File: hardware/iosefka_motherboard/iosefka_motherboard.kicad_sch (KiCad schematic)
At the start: 16 parts, among them J4 Conn_01x10, J9 Conn_01x10, U5 24LC256, U6 Raspberry Pi Pico, U7 MCP3201, U8 MCP4822

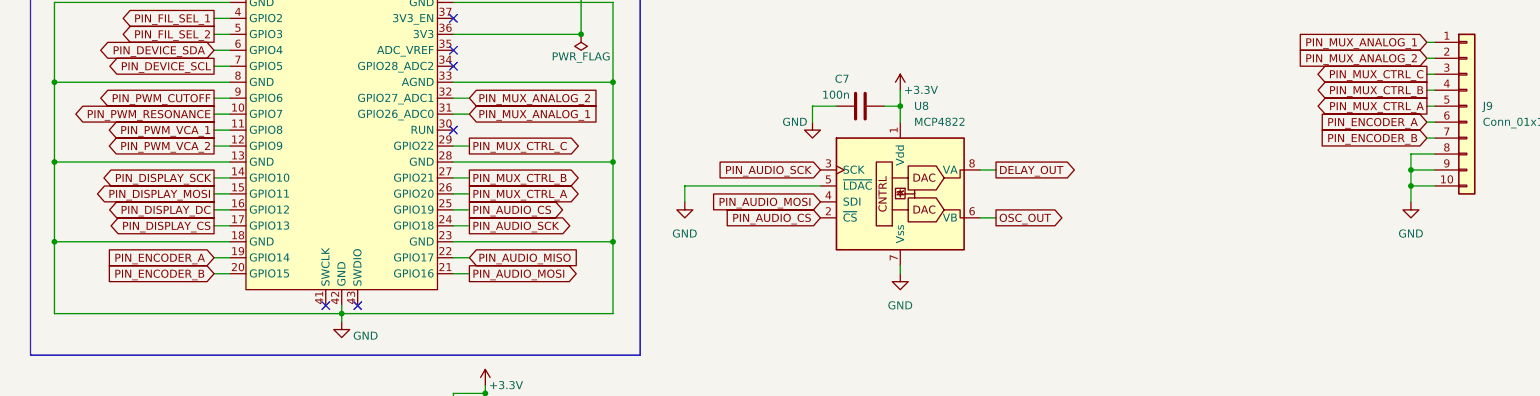
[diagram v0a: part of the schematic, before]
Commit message: added docs
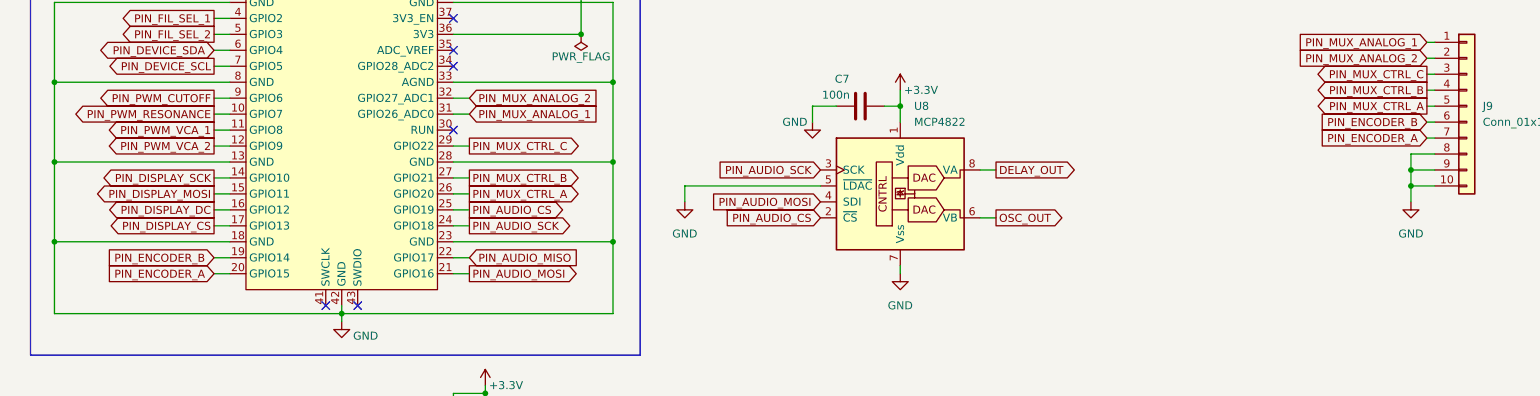
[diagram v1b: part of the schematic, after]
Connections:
- net PIN_ENCODER_A: now also J9.7 (Pin_7), U6.20 (GPIO15); no longer J9.6 (Pin_6), U6.19 (GPIO14)
- net PIN_ENCODER_B: now also J9.6 (Pin_6), U6.19 (GPIO14); no longer J9.7 (Pin_7), U6.20 (GPIO15)
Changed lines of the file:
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@@
+		)
+	)
+	(global_label "PIN_ENCODER_A"
+		(shape input)
+		(at 43.18 110.49 180)
+		(fields_autoplaced yes)
+		(effects
+			(font
+				(size 1.27 1.27)
+			)
+			(justify right)
+		)
+		(property "Intersheetrefs" "${INTERSHEET_REFS}"
+			(at 25.1967 110.49 0)
+			(effects
+				(font
+					(size 1.27 1.27)
+				)
+				(justify right)
+				(hide yes)
+			)
+		)
+	)
+	(global_label "PIN_PWM_VCA_2"
+		(shape output)
+		(at 43.18 90.17 180)
+		(fields_autoplaced yes)
+		(effects
+			(font
+				(size 1.27 1.27)
+			)
+			(justify right)
+		)
+		(property "Intersheetrefs" "${INTERSHEET_REFS}"
+			(at 25.2572 90.17 0)
+			(effects
+				(font
+					(size 1.27 1.27)
+				)
+				(justify right)
+				(hide yes)
+			)
+		)
+	)
+	(global_label "PIN_MUX_ANALOG_1"
+		(shape input)
+		(at 236.22 73.66 180)
+		(fields_autoplaced yes)
+		(effects
+			(font
+				(size 1.27 1.27)
+			)
+			(justify right)
+		)
+		(property "Intersheetrefs" "${INTERSHEET_REFS}"
+			(at 214.7895 73.66 0)
+			(effects
+				(font
+					(size 1.27 1.27)
+				)
+				(justify right)
+				(hide yes)
+			)
+		)
+	)
+	(global_label "PIN_AUDIO_SCK"
+		(shape input)
+		(at 99.06 152.4 0)
+		(fields_autoplaced yes)
+		(effects
+			(font
+				(size 1.27 1.27)
+			)
+			(justify left)
+		)
+		(property "Intersheetrefs" "${INTERSHEET_REFS}"
+			(at 116.5596 152.4 0)
+			(effects
+				(font
+					(size 1.27 1.27)
+				)
+				(justify left)
+				(hide yes)
+			)
+		)
+	)
+	(global_label "PIN_MUX_CTRL_C"
+		(shape output)
+		(at 83.82 90.17 0)
+		(fields_autoplaced yes)
+		(effects
+			(font
+				(size 1.27 1.27)
+			)
+			(justify left)
+		)
+		(property "Intersheetrefs" "${INTERSHEET_REFS}"
+			(at 102.7104 90.17 0)
+			(effects
+				(font
+					(size 1.27 1.27)
+				)
+				(justify left)
+				(hide yes)
+			)
+		)
+	)
+	(global_label "PIN_DEVICE_SCL"
+		(shape output)
+		(at 236.22 62.23 180)
+		(fields_autoplaced yes)
+		(effects
+			(font
+				(size 1.27 1.27)
+			)
+			(justify right)
+		)
+		(property "Intersheetrefs" "${INTERSHEET_REFS}"
+			(at 216.8835 62.23 0)
+			(effects
+				(font
+					(size 1.27 1.27)
+				)
+				(justify right)
+				(hide yes)
+			)
+		)
+	)
+	(global_label "PIN_DISPLAY_CS"
+		(shape output)
+		(at 43.18 102.87 180)
+		(fields_autoplaced yes)
+		(effects
+			(font
+				(size 1.27 1.27)
+			)
+			(justify right)
+		)
+		(property "Intersheetrefs" "${INTERSHEET_REFS}"
+			(at 25.0152 102.87 0)
+			(effects
+				(font
+					(size 1.27 1.27)
+				)
+				(justify right)
+				(hide yes)
+			)
+		)
+	)
+	(global_label "OSC_OUT"
+		(shape output)
+		(at 167.64 101.6 0)
+		(fields_autoplaced yes)
+		(effects
+			(font
+				(size 1.27 1.27)
+			)
+			(justify left)
+		)
+		(property "Intersheetrefs" "${INTERSHEET_REFS}"
+			(at 180.8457 101.6 0)
+			(effects
+				(font
+					(size 1.27 1.27)
+				)
+				(justify left)
+				(hide yes)
+			)
 		)
 	)
 	(global_label "PIN_ENCODER_B"
-		(shape input)
-		(at 43.18 110.49 180)
-		(fields_autoplaced yes)
-		(effects
-			(font
-				(size 1.27 1.27)
-			)
-			(justify right)
-		)
-		(property "Intersheetrefs" "${INTERSHEET_REFS}"
-			(at 25.0153 110.49 0)
-			(effects
-				(font
-					(size 1.27 1.27)
-				)
-				(justify right)
-				(hide yes)
-			)
-		)
-	)
-	(global_label "PIN_PWM_VCA_2"
-		(shape output)
-		(at 43.18 90.17 180)
-		(fields_autoplaced yes)
-		(effects
-			(font
-				(size 1.27 1.27)
-			)
-			(justify right)
-		)
-		(property "Intersheetrefs" "${INTERSHEET_REFS}"
-			(at 25.2572 90.17 0)
-			(effects
-				(font
-					(size 1.27 1.27)
-				)
-				(justify right)
-				(hide yes)
-			)
-		)
-	)
-	(global_label "PIN_MUX_ANALOG_1"
-		(shape input)
-		(at 236.22 73.66 180)
-		(fields_autoplaced yes)
-		(effects
-			(font
-				(size 1.27 1.27)
-			)
-			(justify right)
-		)
-		(property "Intersheetrefs" "${INTERSHEET_REFS}"
-			(at 214.7895 73.66 0)
-			(effects
-				(font
-					(size 1.27 1.27)
-				)
-				(justify right)
-				(hide yes)
-			)
-		)
-	)
-	(global_label "PIN_AUDIO_SCK"
-		(shape input)
-		(at 99.06 152.4 0)
-		(fields_autoplaced yes)
-		(effects
-			(font
-				(size 1.27 1.27)
-			)
-			(justify left)
-		)
-		(property "Intersheetrefs" "${INTERSHEET_REFS}"
-			(at 116.5596 152.4 0)
-			(effects
-				(font
-					(size 1.27 1.27)
-				)
-				(justify left)
-				(hide yes)
-			)
-		)
-	)
-	(global_label "PIN_MUX_CTRL_C"
-		(shape output)
-		(at 83.82 90.17 0)
-		(fields_autoplaced yes)
-		(effects
-			(font
-				(size 1.27 1.27)
-			)
-			(justify left)
-		)
-		(property "Intersheetrefs" "${INTERSHEET_REFS}"
-			(at 102.7104 90.17 0)
-			(effects
-				(font
-					(size 1.27 1.27)
-				)
-				(justify left)
-				(hide yes)
-			)
-		)
-	)
-	(global_label "PIN_DEVICE_SCL"
-		(shape output)
-		(at 236.22 62.23 180)
-		(fields_autoplaced yes)
-		(effects
-			(font
-				(size 1.27 1.27)
-			)
-			(justify right)
-		)
-		(property "Intersheetrefs" "${INTERSHEET_REFS}"
-			(at 216.8835 62.23 0)
-			(effects
-				(font
-					(size 1.27 1.27)
-				)
-				(justify right)
-				(hide yes)
-			)
-		)
-	)
-	(global_label "PIN_DISPLAY_CS"
-		(shape output)
-		(at 43.18 102.87 180)
-		(fields_autoplaced yes)
-		(effects
-			(font
-				(size 1.27 1.27)
-			)
-			(justify right)
-		)
-		(property "Intersheetrefs" "${INTERSHEET_REFS}"
-			(at 25.0152 102.87 0)
-			(effects
-				(font
-					(size 1.27 1.27)
-				)
-				(justify right)
-				(hide yes)
-			)
-		)
-	)
-	(global_label "OSC_OUT"
-		(shape output)
-		(at 167.64 101.6 0)
-		(fields_autoplaced yes)
-		(effects
-			(font
-				(size 1.27 1.27)
-			)
-			(justify left)
-		)
-		(property "Intersheetrefs" "${INTERSHEET_REFS}"
-			(at 180.8457 101.6 0)
-			(effects
-				(font
-					(size 1.27 1.27)
-				)
-				(justify left)
-				(hide yes)
-			)
-		)
-	)
-	(global_label "PIN_ENCODER_A"
 		(shape input)
 		(at 236.22 86.36 180)
@@
 		)
 	)
-	(global_label "PIN_ENCODER_A"
+	(global_label "PIN_ENCODER_B"
 		(shape input)
 		(at 43.18 107.95 180)
@@
 		)
 		(property "Intersheetrefs" "${INTERSHEET_REFS}"
-			(at 25.1967 107.95 0)
+			(at 25.0153 107.95 0)
 			(effects
 				(font
@@
 		)
 	)
-	(global_label "PIN_ENCODER_B"
+	(global_label "PIN_ENCODER_A"
 		(shape input)
 		(at 236.22 88.9 180)
